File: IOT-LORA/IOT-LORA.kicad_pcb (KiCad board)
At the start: 2 copper layers, 36 parts, among them J1 Conn_01x02, J2 Conn_01x06, J3 Conn_01x03, J4 Conn_01x03, J5 Conn_01x03, J6 Conn_01x03, J7 Conn_01x04, J8 Conn_01x04, J9 Conn_01x06, U1 LM1117-3.3, U2 ATmega328-AU, U3 Ai-Thinker-Ra-01, Y1 Crystal_Small

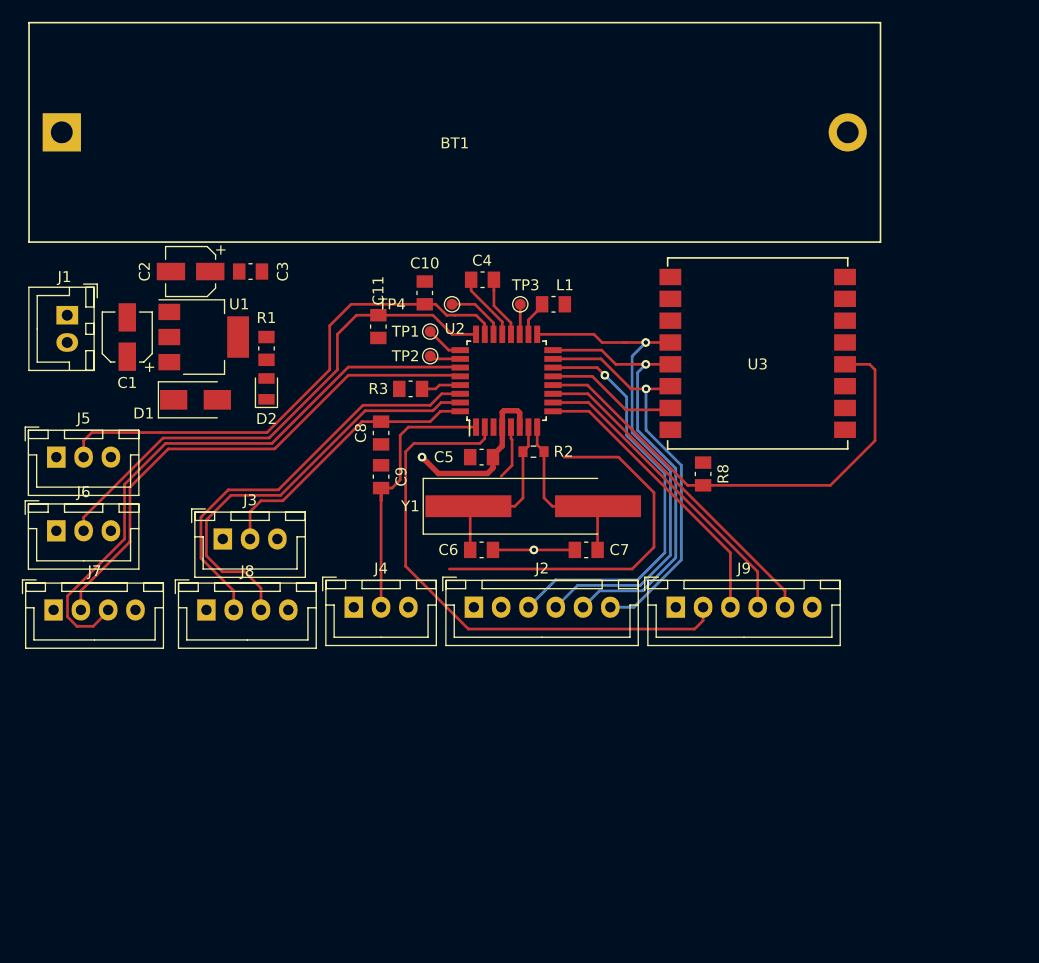
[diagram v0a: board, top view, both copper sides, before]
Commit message: modifier
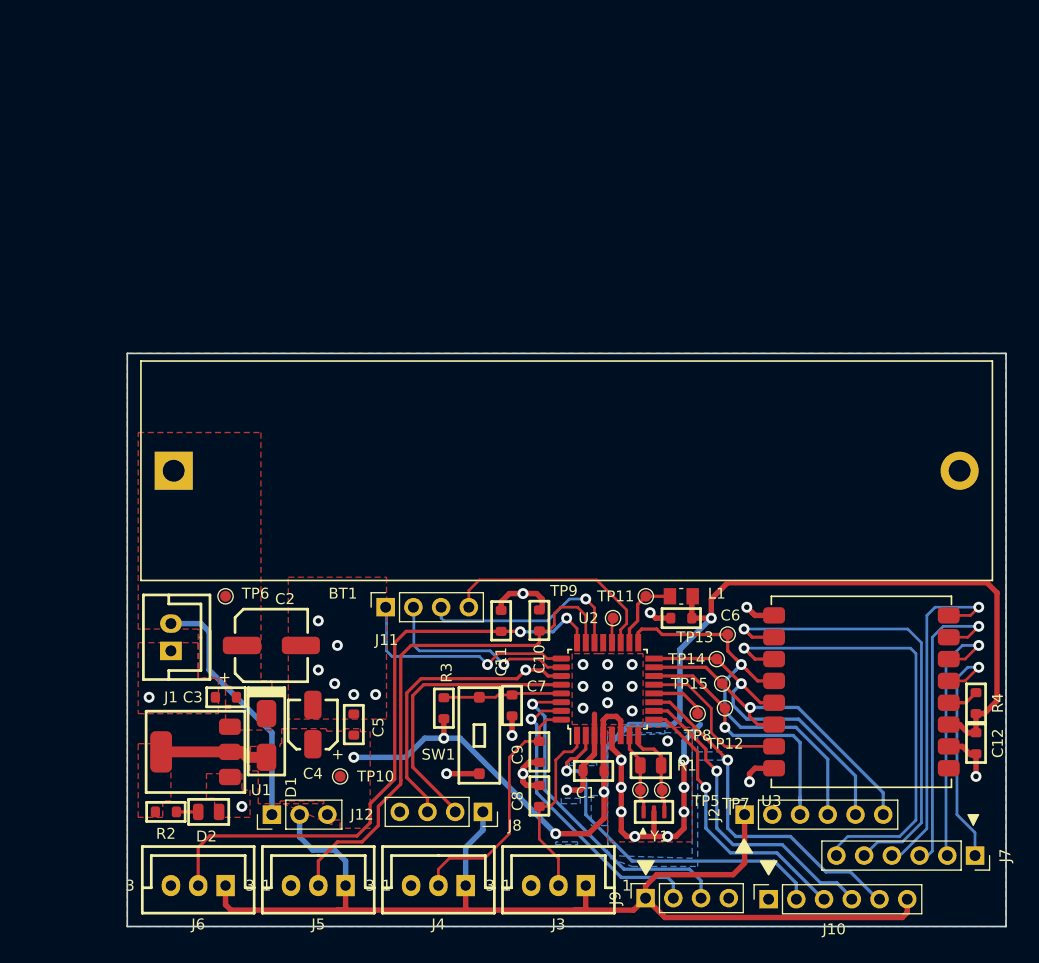
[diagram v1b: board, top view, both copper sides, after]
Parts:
- removed R8: 10k, Resistor_SMD:R_0805_2012Metric_Pad1.15x1.50mm_HandSolder
- removed TP1, TP2, TP3, TP4: Test_Point, TestPoint:TestPoint_Pad_D1.0mm
- added C12: 100n, LEEVAWN:C_0603_1608Metric_Pad0.84x1.00mm_HandSolder_jp, F.Cu at (188.0, 110.5)
- added J11: Conn_01x04, Connector_PinSocket_2.54mm:PinSocket_1x04_P2.54mm_Vertical, F.Cu at (133.9, 98.0)
- added J12: Conn_01x03_Male, Connector_PinHeader_2.54mm:PinHeader_1x03_P2.54mm_Vertical, F.Cu at (123.5, 117.0)
- added J9: Conn_01x04, Connector_PinSocket_2.54mm:PinSocket_1x04_P2.54mm_Vertical, F.Cu at (157.7, 124.7)
- added R4: 10k, LEEVAWN:R_0603_1608Metric_Pad0.84x1.00mm_HandSolder_jp, F.Cu at (188.0, 106.8)
- added SW1: RESET BUTTON, LEEVAWN:EL-3625-W, F.Cu at (142.5, 109.8)
- added TP10: TestPoint, TestPoint:TestPoint_Pad_D1.0mm, F.Cu at (129.8, 113.5)
- added TP11: TestPoint, TestPoint:TestPoint_Pad_D1.0mm, F.Cu at (157.8, 97.0)
- added TP12: TestPoint, TestPoint:TestPoint_Pad_D1.0mm, F.Cu at (165.0, 107.2)
- added TP13: TestPoint, TestPoint:TestPoint_Pad_D1.0mm, F.Cu at (165.2, 100.5)
- added TP14: TestPoint, TestPoint:TestPoint_Pad_D1.0mm, F.Cu at (164.2, 102.8)
- added TP15: TestPoint, TestPoint:TestPoint_Pad_D1.0mm, F.Cu at (164.8, 105.0)
- added TP5: TestPoint, TestPoint:TestPoint_Pad_D1.0mm, F.Cu at (157.2, 114.8)
- added TP6: TestPoint, TestPoint:TestPoint_Pad_D1.0mm, F.Cu at (119.2, 97.0)
- added TP7: TestPoint, TestPoint:TestPoint_Pad_D1.0mm, F.Cu at (159.2, 114.8)
- added TP8: Test_Point, TestPoint:TestPoint_Pad_D1.0mm, F.Cu at (162.5, 107.8)
- added TP9: Test_Point, TestPoint:TestPoint_Pad_D1.0mm, F.Cu at (154.8, 99.0)
- C1: value 10u 16v -> 100n; footprint Capacitor_SMD:CP_Elec_4x5.3 -> LEEVAWN:C_0603_1608Metric_Pad0.84x1.00mm_HandSolder_jp
- C10, C11, C3, C5, C8, C9: footprint Capacitor_SMD:C_0805_2012Metric_Pad1.15x1.50mm_HandSolder -> LEEVAWN:C_0603_1608Metric_Pad0.84x1.00mm_HandSolder_jp
- C2: value 10u 16v -> 100u; footprint Capacitor_SMD:CP_Elec_4x5.3 -> LEEVAWN:CP_Elec_6.3x7.7_jp
- C4: value 100n -> 10u 16v; footprint Capacitor_SMD:C_0805_2012Metric_Pad1.15x1.50mm_HandSolder -> LEEVAWN:CP_Elec_4x5.3_jp
- C6, C7: value C_Small -> 100n; footprint Capacitor_SMD:C_0805_2012Metric_Pad1.15x1.50mm_HandSolder -> LEEVAWN:C_0603_1608Metric_Pad0.84x1.00mm_HandSolder_jp
- D1: value D -> 40V 3A; footprint Diode_SMD:D_SMA -> LEEVAWN:D_SMA
- D2: footprint LED_SMD:LED_0805_2012Metric_Pad0.97x1.50mm_HandSolder -> LEEVAWN:LED_0805_2012Metric_Pad0.97x1.50mm_HandSolder
- J1: footprint Connector_JST:JST_XH_B02B-XH-A_1x02_P2.50mm_Vertical -> LEEVAWN:2P-XH2.54-V
- J10: renamed from J9; footprint Connector_JST:JST_XH_B06B-XH-A_1x06_P2.50mm_Vertical -> Connector_PinSocket_2.54mm:PinSocket_1x06_P2.54mm_Vertical
- J2: value Conn_01x06 -> SPI BUS; footprint Connector_JST:JST_XH_B06B-XH-A_1x06_P2.50mm_Vertical -> Connector_PinSocket_2.54mm:PinSocket_1x06_P2.54mm_Vertical
- J3, J4, J5, J6: footprint Connector_JST:JST_XH_B03B-XH-A_1x03_P2.50mm_Vertical -> LEEVAWN:3P-XH2.54-V
- J7: value Conn_01x04 -> Conn_01x06; footprint Connector_JST:JST_XH_B04B-XH-A_1x04_P2.50mm_Vertical -> Connector_PinSocket_2.54mm:PinSocket_1x06_P2.54mm_Vertical
- J8: footprint Connector_JST:JST_XH_B04B-XH-A_1x04_P2.50mm_Vertical -> Connector_PinSocket_2.54mm:PinSocket_1x04_P2.54mm_Vertical
- R1: value 330 -> 1 M; footprint Resistor_SMD:R_0805_2012Metric_Pad1.15x1.50mm_HandSolder -> LEEVAWN:R_0805_2012Metric_jp
- R2: value 1M -> 330; footprint Resistor_SMD:R_0603_1608Metric_Pad0.84x1.00mm_HandSolder -> LEEVAWN:R_0603_1608Metric_Pad0.84x1.00mm_HandSolder_jp
- R3: footprint Resistor_SMD:R_0805_2012Metric_Pad1.15x1.50mm_HandSolder -> LEEVAWN:R_0603_1608Metric_Pad0.84x1.00mm_HandSolder_jp
- U1: footprint Package_TO_SOT_SMD:SOT-223-3_TabPin2 -> LEEVAWN:SOT-223-3_TabPin2
- U2: value ATmega328-AU -> ATMEGA328P-AU
- U3: footprint RF_Module:Ai-Thinker-Ra-01-LoRa -> LEEVAWN:Ai-Thinker-Ra-01-LoRa
- Y1: value Crystal_Small -> 8Mhz; footprint Crystal:Crystal_SMD_HC49-SD_HandSoldering -> LEEVAWN:CSTNE16M00V2
- moved J7 87.4 mm to (187.9, 120.8), turned to 270 degrees
- moved C1 58.3 mm to (153.0, 113.0), turned to 180 degrees
- moved R1 52.0 mm to (158.2, 112.5), turned to 0 degrees
- moved J5 47.4 mm to (130.2, 123.5), turned to 180 degrees
- moved R2 47.1 mm to (113.8, 116.8)
- moved J3 46.0 mm to (152.2, 123.5), turned to 180 degrees
- moved C4 43.6 mm to (127.2, 108.8), turned to 90 degrees
- moved D2 39.1 mm to (117.7, 116.8), turned to 180 degrees
- moved C3 39.1 mm to (119.3, 106.2), turned to 180 degrees
- moved U1 38.0 mm to (116.5, 111.2), turned to 180 degrees
- moved C8 36.3 mm to (148.0, 115.3), turned to 270 degrees
- moved J6 36.0 mm to (119.2, 123.5), turned to 180 degrees
- moved C2 35.0 mm to (123.5, 101.5), turned to 0 degrees
- moved BT1 32.7 mm to (114.5, 85.5)
- moved U3 32.4 mm to (177.5, 105.8)
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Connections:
- BT1 pad 1: VCC_5V -> +5V
- BT1 pad 2: GND_5V -> GND
- C1 pad 1: VCC_5V -> +3V3
- C1 pad 2: GND_5V -> GND
- C10 pad 1: GND_5V -> GND
- C11 pad 1: GND_5V -> GND
- C2 pad 1: +3V3 -> +5V
- C2 pad 2: GND_5V -> GND
- C3 pad 1: +3V3 -> +5V
- C3 pad 2: GND_5V -> GND
- C4 pad 1: GND_5V -> +3V3
- C4 pad 2: Net-(C4-Pad2) -> GND
- C5 pad 2: (no net) -> GND
- C6 pad 1: Net-(C6-Pad1) -> GND
- C6 pad 2: Net-(C6-Pad2) -> +3V3
- C7 pad 1: Net-(C6-Pad1) -> GND
- C7 pad 2: Net-(C7-Pad2) -> RS
- C8 pad 1: GND_5V -> GND
- C8 pad 2: SIG2 -> SIG3
- C9 pad 1: GND_5V -> GND
- C9 pad 2: SIG3 -> SIG2
- D1 pad 1: VCC_5V -> +5V
- D2 pad 1: GND_5V -> GND
- J1 pad 1: GND_5V -> GND
- J1 pad 2: VCC_5V -> +5V
- J3 pad 2: SIG2 -> SIG3
- J4 pad 2: SIG3 -> SIG2
- J7 pad 1: VCC -> Net-(J7-Pad1)
- J7 pad 2: SCL -> Net-(J7-Pad2)
- J7 pad 3: SDA -> Net-(J7-Pad3)
- J7 pad 4: GND -> Net-(J7-Pad4)
- J8 pad 2: TX -> SCL
- J8 pad 3: RX -> SDA
- L1 pad 1: +3V3 -> Net-(L1-Pad1)
- L1 pad 2: Net-(L1-Pad2) -> +3V3
- R1 pad 1: +3V3 -> Net-(R1-Pad1)
- R1 pad 2: Net-(D2-Pad2) -> Net-(R1-Pad2)
- R2 pad 1: Net-(C6-Pad2) -> +3V3
- R2 pad 2: Net-(C7-Pad2) -> Net-(D2-Pad2)
- R3 pad 2: Net-(R3-Pad2) -> RS
- U1 pad 1: GND_5V -> GND
- U1 pad 3: VCC_5V -> +5V
- U2 pad 12: RS -> Net-(TP8-Pad1)
- U2 pad 18: Net-(L1-Pad2) -> Net-(L1-Pad1)
- U2 pad 20: Net-(C4-Pad2) -> Net-(TP9-Pad1)
- U2 pad 21: GND_5V -> (no net)
- U2 pad 29: Net-(R3-Pad2) -> RS
- U2 pad 3: GND_5V -> GND
- U2 pad 30: TX -> RX
- U2 pad 31: RX -> TX
- U2 pad 5: GND_5V -> GND
- U2 pad 7: Net-(C6-Pad2) -> Net-(R1-Pad1)
- U2 pad 8: Net-(C7-Pad2) -> Net-(R1-Pad2)
- U3 pad 10: (no net) -> Net-(J7-Pad5)
- U3 pad 11: (no net) -> Net-(J7-Pad6)
- U3 pad 16: GND_5V -> GND
- U3 pad 2: GND_5V -> GND
- U3 pad 4: RS -> Net-(R4-Pad2)
- U3 pad 5: (no net) -> Net-(J7-Pad1)
- U3 pad 6: (no net) -> Net-(J7-Pad2)
- U3 pad 7: (no net) -> Net-(J7-Pad3)
- U3 pad 8: (no net) -> Net-(J7-Pad4)
- U3 pad 9: GND_5V -> GND
- Y1 pad 1: Net-(C6-Pad2) -> Net-(R1-Pad1)
- Y1 pad 2: Net-(C7-Pad2) -> GND
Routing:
- net +3V3: track 15.8 -> 123.7 mm, vias 1 -> 5
- net VCC: track 0.00 -> 107.8 mm
- net GND: track 0.00 -> 65.0 mm, vias 0 -> 35
- net GND_5V: track 45.3 -> 0.00 mm
- net Net-(J7-Pad6): track 0.00 -> 44.2 mm, vias 0 -> 1
- net Net-(J7-Pad5): track 0.00 -> 43.6 mm, vias 0 -> 1
- net RS: track 44.5 -> 11.0 mm
- net Net-(J7-Pad4): track 0.00 -> 32.2 mm, vias 0 -> 1
- net Net-(J7-Pad3): track 0.00 -> 29.1 mm, vias 0 -> 1
- net SDA: track 54.3 -> 26.9 mm, vias 0 -> 1
- net Net-(J7-Pad2): track 0.00 -> 25.4 mm, vias 0 -> 1
- net Net-(J7-Pad1): track 0.00 -> 23.4 mm, vias 0 -> 1
- net +5V: track 0.00 -> 22.9 mm
- net SCL: track 47.7 -> 26.3 mm
- net SIGA6: track 2.77 -> 20.8 mm
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- added copper zone on F.Cu, net +3V3
- added copper zone on F.Cu, net +5V
- added copper zone on B.Cu, net GND
- added copper zone on F.Cu, net GND
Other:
- board outline added: 80.5 x 52.5 mm
- net class 0.5 MM added: clearance 0.5, trace_width 0.5, via_dia 1, via_drill 0.5
- net class Default: via_dia 0.8 -> 1; via_drill 0.4 -> 0.5
- board text added: "+5V"
- board text added: "LORA STATION V1"
